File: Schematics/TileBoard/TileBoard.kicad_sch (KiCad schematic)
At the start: 24 parts, among them J1 Input, J2 Power, J3 Output, J4 Prog, SW1 LUT, SW2 RST, U1 74LS251, U2 ATSAMD09D14A-M

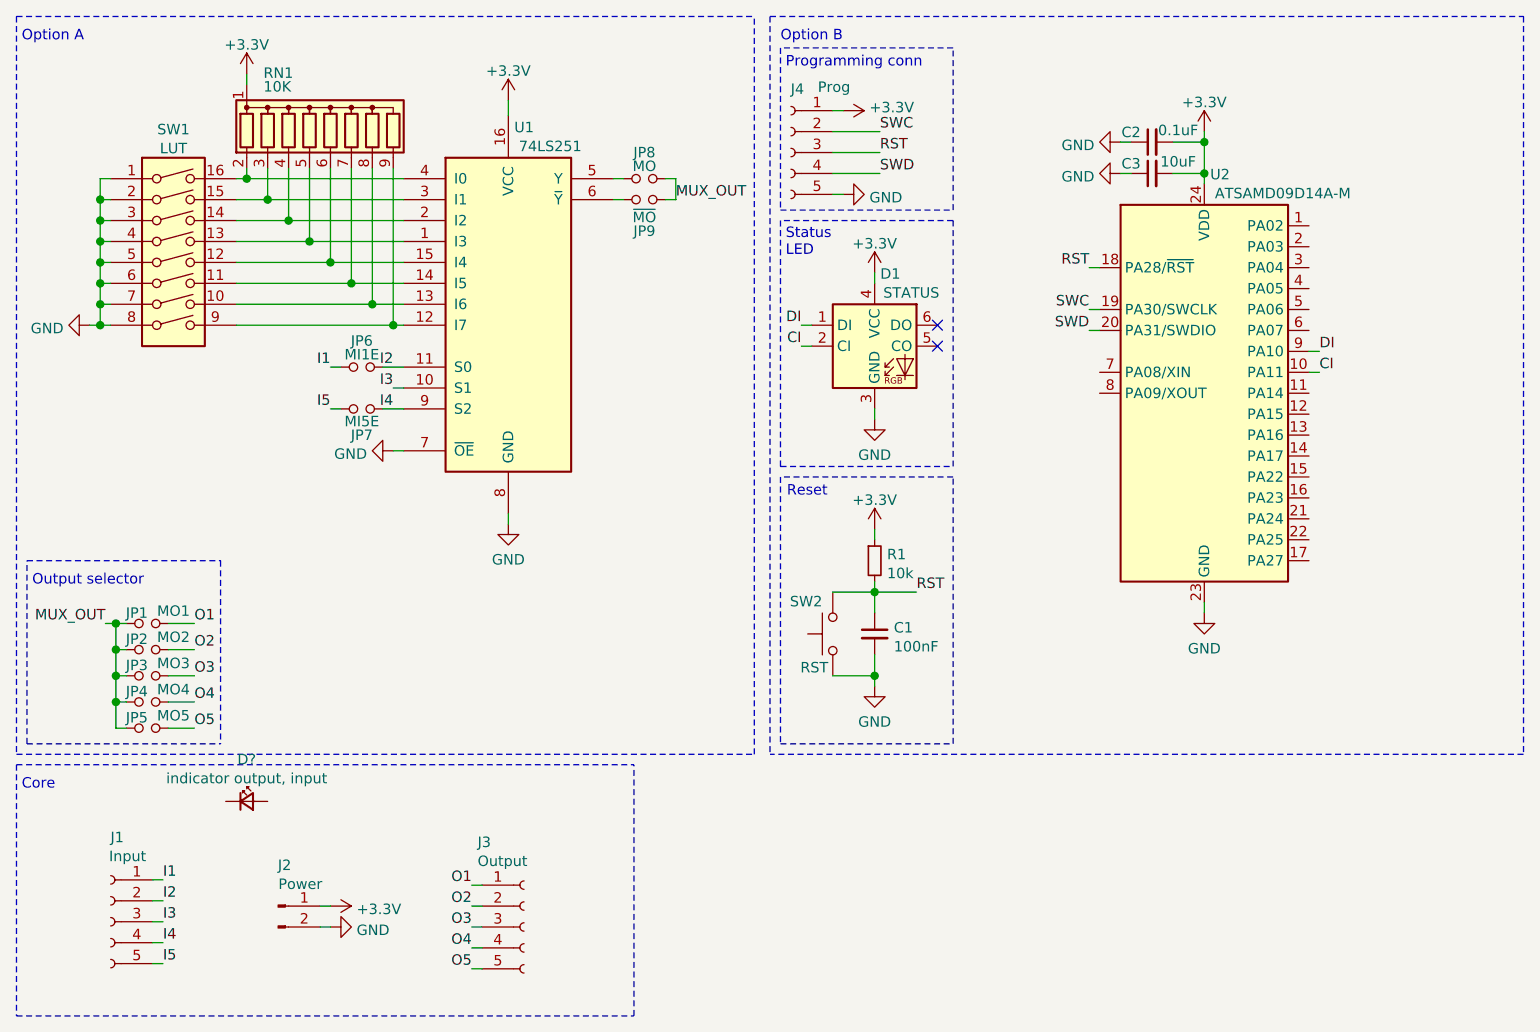
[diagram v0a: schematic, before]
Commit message: TileBoard completed
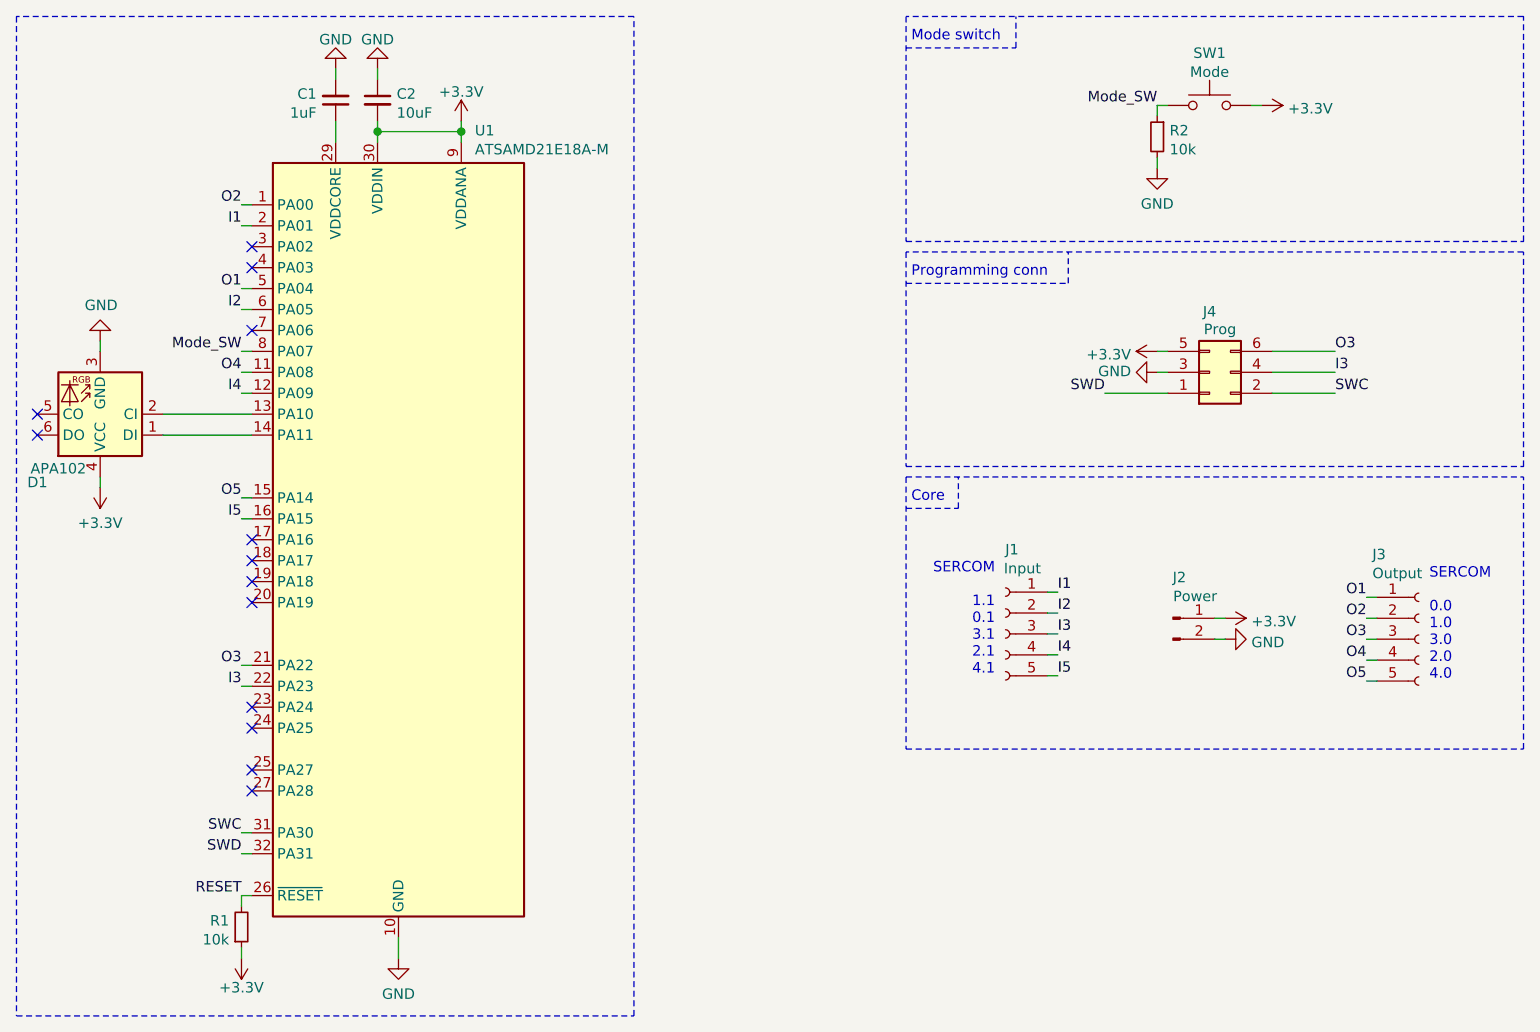
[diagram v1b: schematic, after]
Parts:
- removed C3: 10uF, Capacitor_SMD:C_0603_1608Metric, symbol Device:C_Small
- removed D?: indicator output, input, symbol Device:LED_Small
- removed J4: Prog, Connector_PinSocket_2.54mm:PinSocket_1x05_P2.54mm_Vertical, symbol Connector:Conn_01x05_Female
- removed JP1: MO1, Jumper:SolderJumper-2_P1.3mm_Open_Pad1.0x1.5mm, symbol Device:Jumper_NO_Small
- removed JP2: MO2, Jumper:SolderJumper-2_P1.3mm_Open_Pad1.0x1.5mm, symbol Device:Jumper_NO_Small
- removed JP3: MO3, Jumper:SolderJumper-2_P1.3mm_Open_Pad1.0x1.5mm, symbol Device:Jumper_NO_Small
- removed JP4: MO4, Jumper:SolderJumper-2_P1.3mm_Open_Pad1.0x1.5mm, symbol Device:Jumper_NO_Small
- removed JP5: MO5, Jumper:SolderJumper-2_P1.3mm_Open_Pad1.0x1.5mm, symbol Device:Jumper_NO_Small
- removed JP6: MI1E, Jumper:SolderJumper-2_P1.3mm_Open_Pad1.0x1.5mm, symbol Device:Jumper_NO_Small
- removed JP7: MI5E, Jumper:SolderJumper-2_P1.3mm_Open_Pad1.0x1.5mm, symbol Device:Jumper_NO_Small
- removed JP8: MO, Jumper:SolderJumper-2_P1.3mm_Open_Pad1.0x1.5mm, symbol Device:Jumper_NO_Small
- removed JP9: ~MO, Jumper:SolderJumper-2_P1.3mm_Open_Pad1.0x1.5mm, symbol Device:Jumper_NO_Small
- removed RN1: 10K, Resistor_THT:R_Array_SIP9, symbol Device:R_Network08
- removed SW1: LUT, symbol Switch:SW_DIP_x08
- removed SW2: RST, symbol Switch:SW_Push
- removed U1: 74LS251, symbol 74xx:74LS251
- removed U2: ATSAMD09D14A-M, Package_DFN_QFN:QFN-24-1EP_4x4mm_P0.5mm_EP2.6x2.6mm, symbol MCU_Microchip_SAMD:ATSAMD09D14A-M
- added J4: Prog, Connector:Tag-Connect_TC2030-IDC-NL_2x03_P1.27mm_Vertical, symbol Connector_Generic:Conn_02x03_Odd_Even
- added R2: 10k, Resistor_SMD:R_0603_1608Metric, symbol Device:R_Small
- added SW1: Mode, Button_Switch_SMD:SW_Push_SPST_NO_Alps_SKRK, symbol Switch:SW_Push
- added U1: ATSAMD21E18A-M, Package_DFN_QFN:QFN-32-1EP_5x5mm_P0.5mm_EP3.6x3.6mm, symbol MCU_Microchip_SAMD:ATSAMD21E18A-M
- C1: value 100nF -> 1uF
- C2: value 0.1uF -> 10uF
- D1: value STATUS -> APA102
- J2: footprint Connector_PinSocket_2.54mm:PinSocket_1x02_P2.54mm_Vertical -> InvertedSwitch:Cherry_MX_PCB_Form
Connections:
- net +3V3: now also J4.5 (Pin_5), SW1.1, U1.30 (VDDIN), U1.9 (VDDANA)
- net GND: now also J4.3 (Pin_3), R2.2, U1.10 (GND), U1.28 (GND)
- net I1: now also U1.2 (PA01)
- net I2: now also U1.6 (PA05)
- net I3: now also J4.4 (Pin_4), U1.22 (PA23)
- net I4: now also U1.12 (PA09)
- net I5: now also U1.16 (PA15)
- net O1: now also U1.5 (PA04)
- net O2: now also U1.1 (PA00)
- net O3: now also J4.6 (Pin_6), U1.21 (PA22)
- net O4: now also U1.11 (PA08)
- net O5: now also U1.15 (PA14)
- net SWC: now also J4.2 (Pin_2), U1.31 (PA30)
- net SWD: now also J4.1 (Pin_1), U1.32 (PA31)
- net CI: no longer names the net of D1.2 (CI)
- net CI: now also U1.13 (PA10)
- net DI: no longer names the net of D1.1 (DI)
- net DI: now also U1.14 (PA11)
- net RST: no longer names the net of C1.1
- net RST: now also U1.29 (VDDCORE); no longer R1.2
- new net Mode_SW: R2.1, SW1.2, U1.8 (PA07)
- new net RESET: R1.2, U1.26 (~RESET)
- no-connect marks 2 -> 13
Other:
- note added: "Mode switch"
- note added: "SERCOM 0.0 1.0 3.0 2.0 4.0"
- note added: "SERCOM 1.1 0.1 3.1 2.1 4.1"
- note removed: "Option A"
- note removed: "Option B"
- note removed: "Output selector"
- note removed: "Reset"
- note removed: "Status LED"
- title: (none) -> TileBoard
- moved on the sheet: J1, J2, J3
